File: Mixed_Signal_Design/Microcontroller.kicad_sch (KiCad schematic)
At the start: 15 parts, among them SW1 RESET, U3 ATmega32A-A, Y1 16MHz

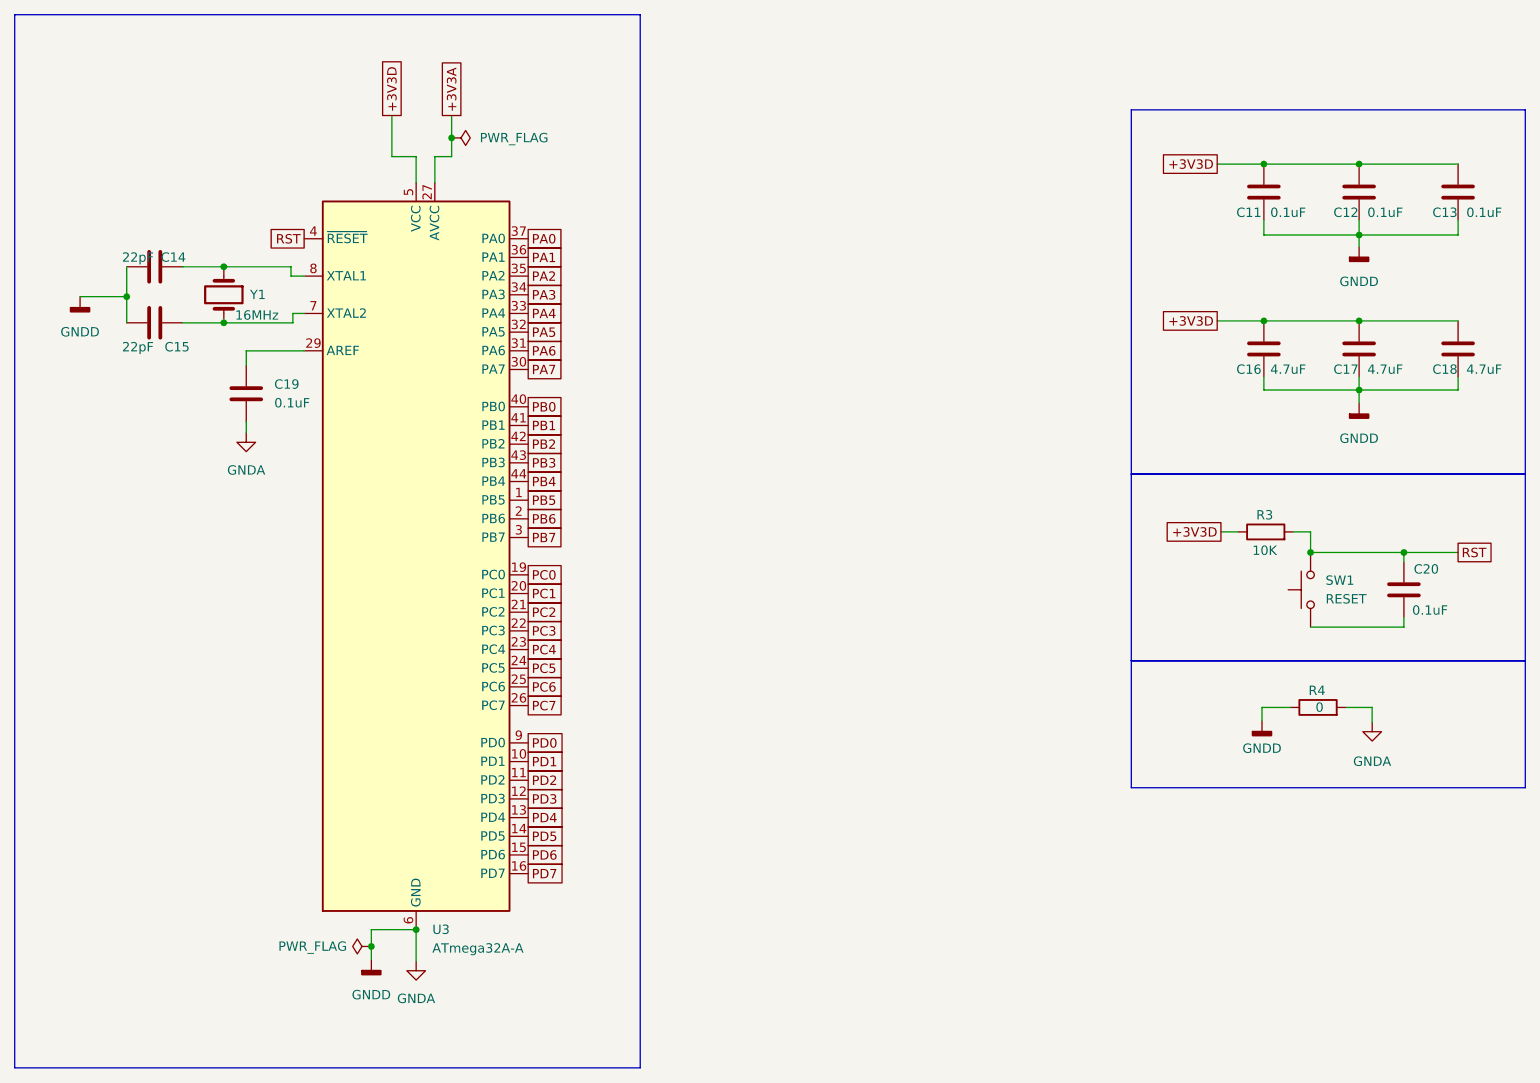
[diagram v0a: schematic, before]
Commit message: commit
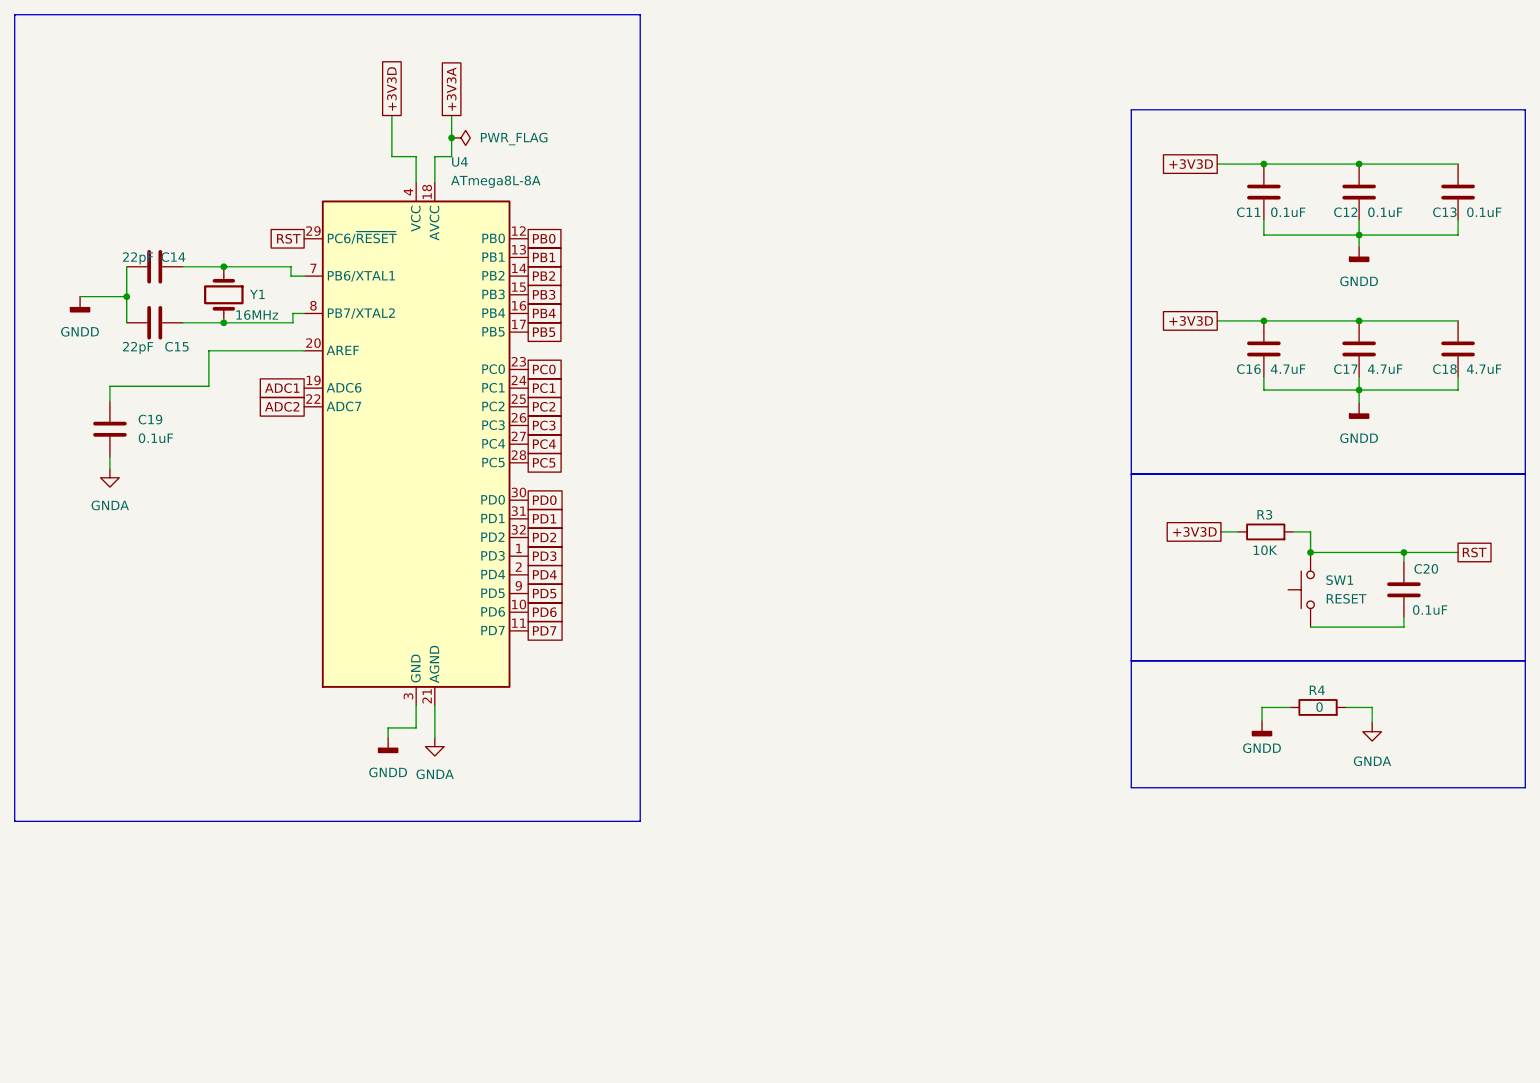
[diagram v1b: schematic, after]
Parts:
- removed U3: ATmega32A-A, Package_QFP:TQFP-44_10x10mm_P0.8mm, symbol MCU_Microchip_ATmega:ATmega32A-A
- added U4: ATmega8L-8A, Package_QFP:TQFP-32_7x7mm_P0.8mm, symbol MCU_Microchip_ATmega:ATmega8L-8A
- C11, C12, C13, C16, C17, C18, C19, C20: footprint (none) -> SparkFun-Capacitor:C_0603_1608Metric
- C14, C15: footprint (none) -> SparkFun-Capacitor:C_0402_1005Metric
- R3, R4: footprint (none) -> Resistor_SMD:R_0402_1005Metric_Pad0.72x0.64mm_HandSolder
- Y1: footprint (none) -> Crystal:Crystal_SMD_HC49-SD
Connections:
- net +3V3A: now also U4.18 (AVCC)
- net +3V3D: now also U4.4 (VCC), U4.6 (VCC)
- net GNDA: now also U4.21 (AGND); no longer C11.2, C12.2, C13.2, C14.1, C15.2, C16.2, C17.2, C18.2, R4.1
- net PB0: now also U4.12 (PB0)
- net PB1: now also U4.13 (PB1)
- net PB2: now also U4.14 (PB2)
- net PB3: now also U4.15 (PB3)
- net PB4: now also U4.16 (PB4)
- net PB5: now also U4.17 (PB5)
- net PC0: now also U4.23 (PC0)
- net PC1: now also U4.24 (PC1)
- net PC2: now also U4.25 (PC2)
- net PC3: now also U4.26 (PC3)
- net PC4: now also U4.27 (PC4)
- net PC5: now also U4.28 (PC5)
- net PD0: now also U4.30 (PD0)
- net PD1: now also U4.31 (PD1)
- net PD2: now also U4.32 (PD2)
- net PD3: now also U4.1 (PD3)
- net PD4: now also U4.2 (PD4)
- net PD5: now also U4.9 (PD5)
- net PD6: now also U4.10 (PD6)
- net PD7: now also U4.11 (PD7)
- net RST: now also U4.29 (PC6/~{RESET})
- net at C14.2, Y1.1: now also U4.7 (PB6/XTAL1)
- net at C15.1, Y1.2: now also U4.8 (PB7/XTAL2)
- net at C19.2: now also U4.20 (AREF)
- new net ADC1: U4.19 (ADC6)
- new net ADC2: U4.22 (ADC7)
- new net GNDD: C11.2, C12.2, C13.2, C14.1, C15.2, C16.2, C17.2, C18.2, R4.1, U4.3 (GND), U4.5 (GND)
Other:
- moved on the sheet: C19
